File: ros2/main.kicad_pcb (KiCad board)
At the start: 2 copper layers, 53 parts, among them J1 Battery Conn_01x02, J2 BMS_input, J3 BMS_output, J5 SW_CONNECTOR, J6 ACS_IN, J7 ACS_POWER_OUT, U2 TB6612NFG, U3 TB6612NFG, U4 TB6612NFG, U5 TB6612NFG, U6 TXS0108E, U7 ACS712_MODULE, U8 XL63070

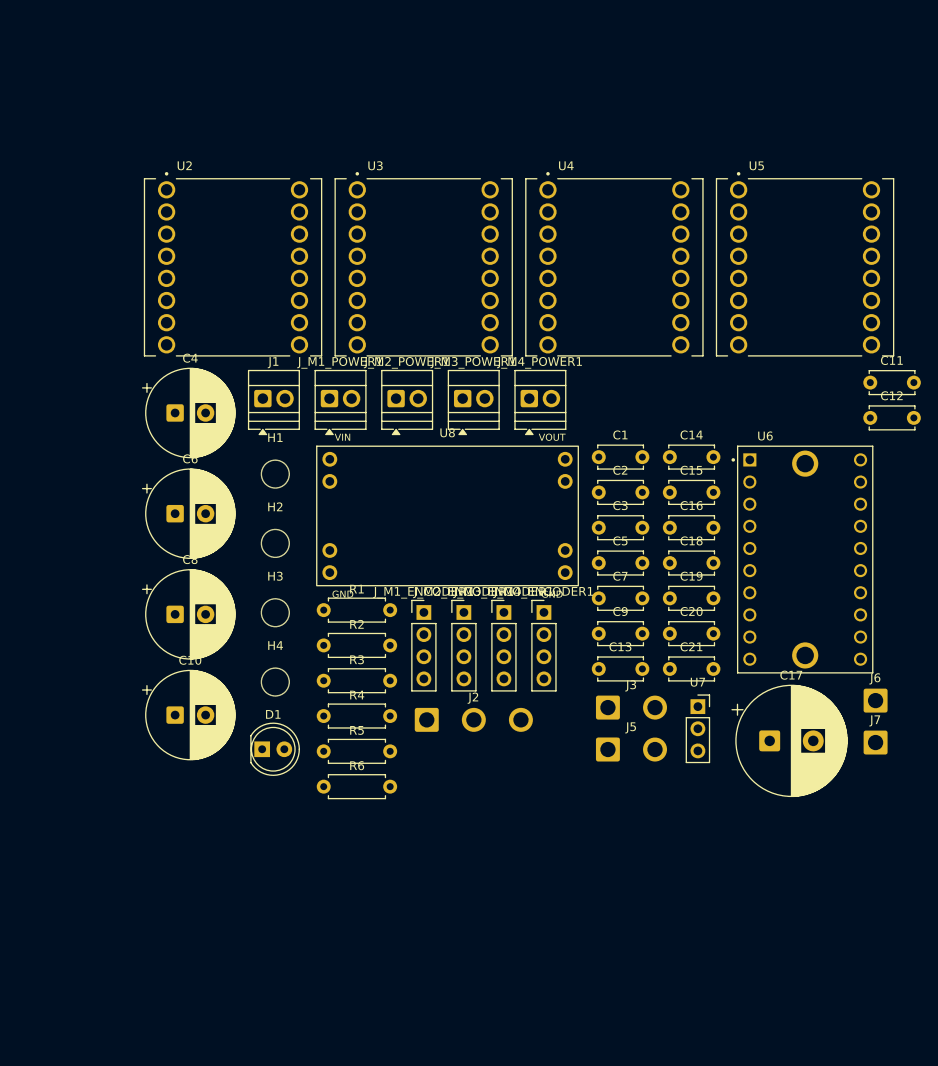
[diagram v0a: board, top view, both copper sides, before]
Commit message: routed pcb + corrected schematic
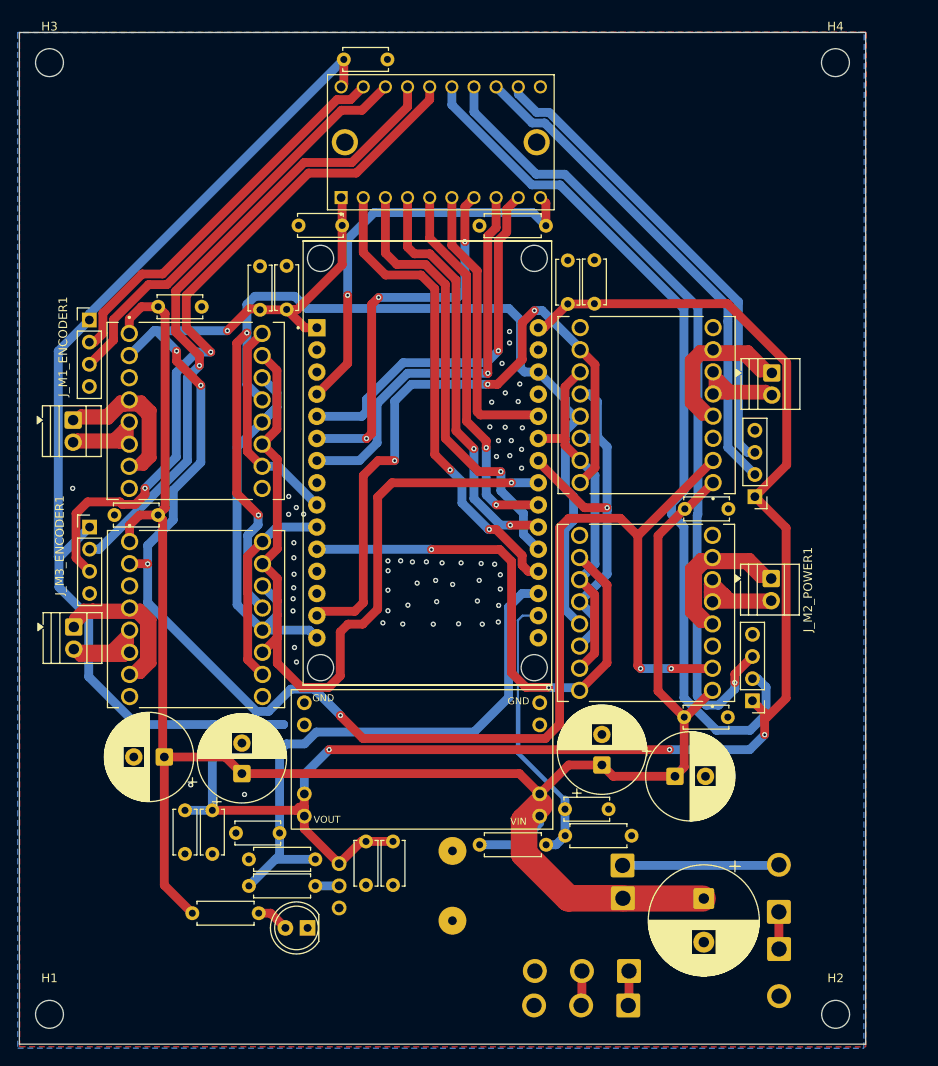
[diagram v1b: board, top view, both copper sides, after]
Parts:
- removed J1: Battery Conn_01x02, TerminalBlock:TerminalBlock_Xinya_XY308-2.54-2P_1x02_P2.54mm_Horizontal
- added J4: Conn_01x03, Connector_Wire:SolderWire-1sqmm_1x03_P5.4mm_D1.4mm_OD2.7mm, F.Cu at (175.4, 128.0)
- added U1: ESP32-DEVKIT-V1, esp32:MODULE_ESP32_DEVKIT_V1, F.Cu at (152.3, 69.7)
- C3, C5, C7, C9: value 22nF -> 100nF
- U7: footprint Connector_PinSocket_2.54mm:PinSocket_1x03_P2.54mm_Vertical -> ACS712_MODULE:ACS712_module
- moved H4 95.8 mm to (199.1, 23.8)
- moved H2 84.0 mm to (199.2, 133.0)
- moved U5 71.8 mm to (125.8, 63.8)
- moved C18 68.8 mm to (142.7, 23.4)
- moved H3 68.2 mm to (109.0, 23.8)
- moved H1 67.2 mm to (109.0, 133.0)
- moved C15 66.5 mm to (124.5, 109.6), turned to -90 degrees
- moved C6 64.8 mm to (180.7, 105.7)
- moved U6 63.5 mm to (153.9, 32.9), turned to 90 degrees
- moved C9 62.9 mm to (121.4, 51.8)
- moved C16 61.7 mm to (127.7, 109.6), turned to -90 degrees
- moved R3 58.1 mm to (165.9, 42.5), turned to 180 degrees
- moved C19 56.9 mm to (142.6, 42.5), turned to 180 degrees
- moved C14 54.3 mm to (148.4, 113.1), turned to -90 degrees
- moved C8 51.9 mm to (172.3, 104.4), turned to 90 degrees
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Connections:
- J2 pad 3: /BAT_RAW_MINUS -> GNDD
- J_M1_ENCODER1 pad 2: GNDD -> /M1_ENC_A
- J_M1_ENCODER1 pad 3: /M1_ENC_A -> /M1_ENC_B
- J_M1_ENCODER1 pad 4: /M1_ENC_B -> GNDD
- J_M2_ENCODER1 pad 2: GNDD -> /M3_ENC_A
- J_M2_ENCODER1 pad 3: /M3_ENC_A -> /M3_ENC_B
- J_M2_ENCODER1 pad 4: /M3_ENC_B -> GNDD
- J_M3_ENCODER1 pad 2: GNDD -> /M2_ENC_A
- J_M3_ENCODER1 pad 3: /M2_ENC_A -> /M2_ENC_B
- J_M3_ENCODER1 pad 4: /M2_ENC_B -> GNDD
- J_M4_ENCODER1 pad 2: GNDD -> /M4_ENC_A
- J_M4_ENCODER1 pad 3: /M4_ENC_A -> /M4_ENC_B
- J_M4_ENCODER1 pad 4: /M4_ENC_B -> GNDD
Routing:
- net +5V: track 0.00 -> 306.2 mm, vias 0 -> 3
- net /POWER+: track 0.00 -> 227.4 mm
- net +3.3V: track 0.00 -> 204.2 mm, vias 0 -> 7
- net /MOTORS_STBY: track 0.00 -> 120.4 mm, vias 0 -> 2
- net /M3_ENC_A: track 0.00 -> 101.0 mm
- net /M3_ENC_B: track 0.00 -> 92.6 mm, vias 0 -> 1
- net /LEFT_IN2: track 0.00 -> 92.5 mm, vias 0 -> 1
- net /M2_ENC_B: track 0.00 -> 83.1 mm, vias 0 -> 2
- net /M4_PWM: track 0.00 -> 78.3 mm, vias 0 -> 3
- net /M2_ENC_A: track 0.00 -> 74.2 mm, vias 0 -> 1
- net /ACS_ESP: track 0.00 -> 64.8 mm
- net /M3_PWM: track 0.00 -> 62.7 mm, vias 0 -> 2
- net /M4_ENC_A: track 0.00 -> 57.6 mm
- net /M1_ENC_A_ESP: track 0.00 -> 54.8 mm, vias 0 -> 2
- net /M4_ENC_B: track 0.00 -> 54.5 mm
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- added copper zone on B.Cu, net GNDD
- added copper zone on F.Cu, net GNDD
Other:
- board outline added: 97.1 x 116 mm
